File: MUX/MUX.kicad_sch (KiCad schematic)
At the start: 104 parts, among them P1 Conn_02x36_Top_Bottom, P2 DB9_Male, P3 DB9_Male, P4 DB9_Male, P5 DB9_Male

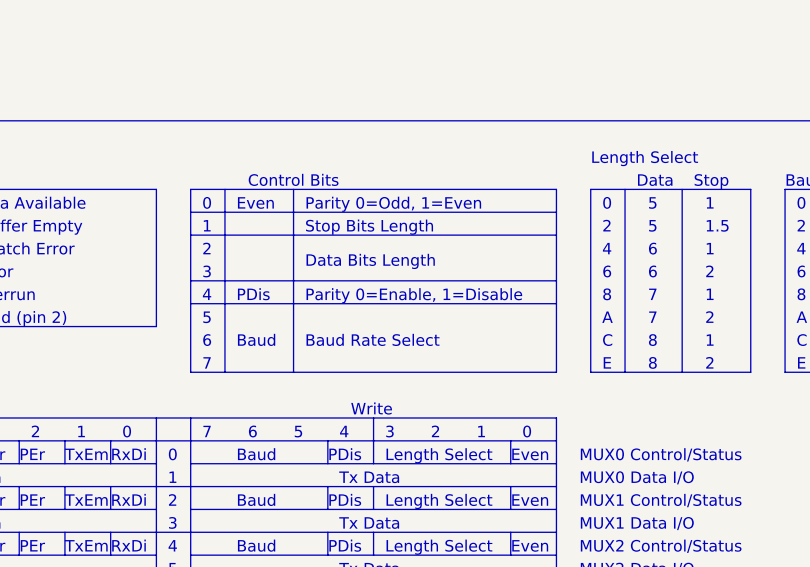
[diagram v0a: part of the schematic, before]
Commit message: misc readability, fix MUX errata
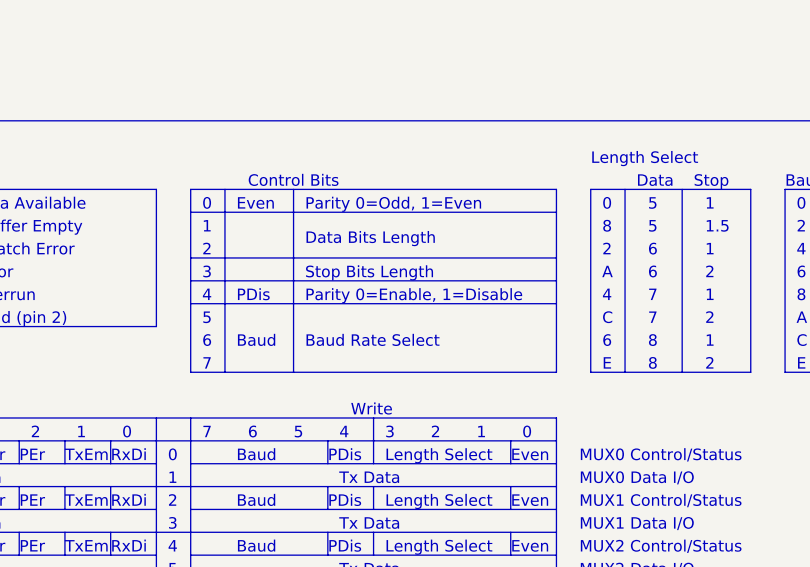
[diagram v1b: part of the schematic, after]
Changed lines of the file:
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@@
   (title_block
     (title "Centurion - 4 Port MUX (Serial Multiplex) Card")
-    (date "2022-09-25")
-    (rev "1.1")
+    (date "2023-05-03")
+    (rev "1.2")
     (company "Meisaka Yukara")
     (comment 1 "Visually Reverse Engineered")
@@
     (stroke (width 0) (type default) (color 0 0 0 0))
   )
-  (polyline (pts (xy 946.15 402.59) (xy 905.51 402.59))
+  (polyline (pts (xy 946.15 405.13) (xy 905.51 405.13))
     (stroke (width 0) (type solid) (color 0 0 0 0))
   )
@@
     (effects (font (size 1.27 1.27)) (justify left bottom))
   )
-  (text "C" (at 951.23 415.29 0)
+  (text "6" (at 951.23 415.29 0)
     (effects (font (size 1.27 1.27)) (justify left bottom))
   )
@@
     (effects (font (size 1.27 1.27)) (justify left bottom))
   )
-  (text "8" (at 951.23 410.21 0)
+  (text "4" (at 951.23 410.21 0)
     (effects (font (size 1.27 1.27)) (justify left bottom))
   )
@@
     (effects (font (size 1.27 1.27)) (justify left bottom))
   )
-  (text "6" (at 951.23 407.67 0)
+  (text "A" (at 951.23 407.67 0)
     (effects (font (size 1.27 1.27)) (justify left bottom))
   )
@@
     (effects (font (size 1.27 1.27)) (justify left bottom))
   )
-  (text "Data Bits Length" (at 918.21 406.4 0)
+  (text "Data Bits Length" (at 918.21 403.86 0)
     (effects (font (size 1.27 1.27)) (justify left bottom))
   )
@@
     (effects (font (size 1.27 1.27)) (justify left bottom))
   )
-  (text "2" (at 951.23 402.59 0)
+  (text "8" (at 951.23 402.59 0)
     (effects (font (size 1.27 1.27)) (justify left bottom))
   )
@@
     (effects (font (size 1.27 1.27)) (justify left bottom))
   )
-  (text "4" (at 951.23 405.13 0)
+  (text "2" (at 951.23 405.13 0)
     (effects (font (size 1.27 1.27)) (justify left bottom))
   )
-  (text "A" (at 951.23 412.75 0)
+  (text "C" (at 951.23 412.75 0)
     (effects (font (size 1.27 1.27)) (justify left bottom))
   )
@@
     (effects (font (size 1.27 1.27)) (justify left bottom))
   )
-  (text "Stop Bits Length" (at 918.21 402.59 0)
+  (text "Stop Bits Length" (at 918.21 407.67 0)
     (effects (font (size 1.27 1.27)) (justify left bottom))
   )
